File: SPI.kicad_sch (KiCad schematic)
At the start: 1 part, among them J14 Conn_01x08

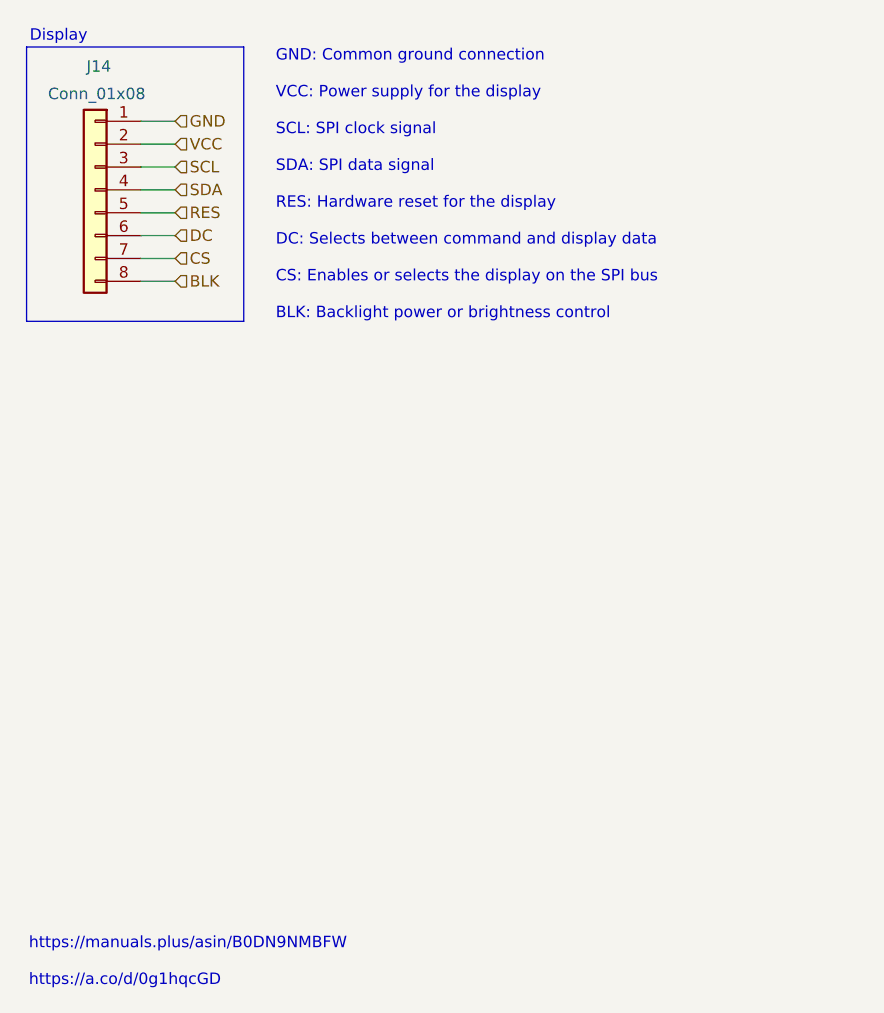
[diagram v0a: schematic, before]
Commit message: org stuf
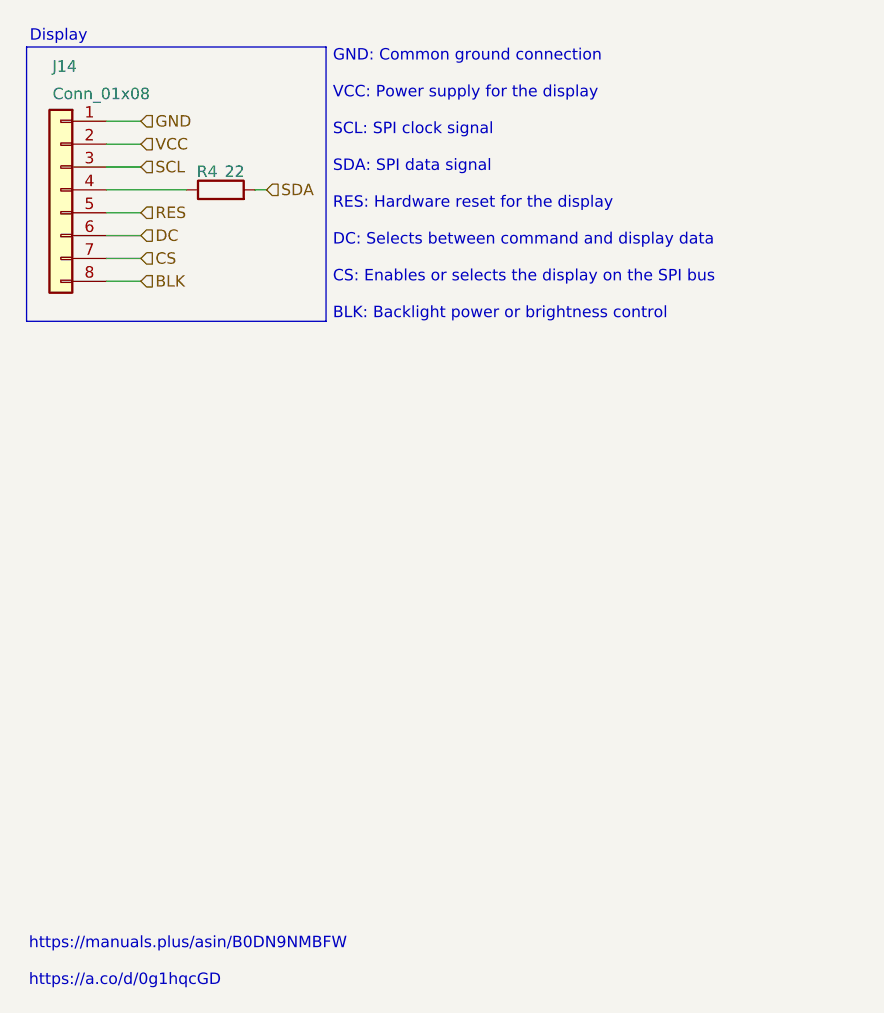
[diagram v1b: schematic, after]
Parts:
- added R4: 22, symbol Device:R
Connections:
- net SDA: now also R4.2; no longer J14.4 (Pin_4)
- new net: J14.4 (Pin_4), R4.1
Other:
- moved on the sheet: J14
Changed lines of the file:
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@@
 	(rectangle
 		(start 15.24 15.875)
-		(end 39.37 46.355)
+		(end 48.514 46.355)
 		(stroke
 			(width 0)
@@
 	(text "GND: Common ground connection\n\nVCC: Power supply for the display\n\nSCL: SPI clock signal\n\nSDA: SPI data signal\n\nRES: Hardware reset for the display\n\nDC: Selects between command and display data\n\nCS: Enables or selects the display on the SPI bus\n\nBLK: Backlight power or brightness control"
 		(exclude_from_sim no)
-		(at 42.926 31.242 0)
+		(at 49.276 31.242 0)
 		(effects
 			(font
@@
 	(wire
 		(pts
-			(xy 27.94 29.21) (xy 31.75 29.21)
+			(xy 24.13 29.21) (xy 27.94 29.21)
 		)
 		(stroke
@@
 	(wire
 		(pts
-			(xy 27.94 24.13) (xy 31.75 24.13)
+			(xy 24.13 24.13) (xy 27.94 24.13)
 		)
 		(stroke
@@
 	(wire
 		(pts
-			(xy 27.94 34.29) (xy 31.75 34.29)
+			(xy 24.13 34.29) (xy 27.94 34.29)
 		)
 		(stroke
@@
 	(wire
 		(pts
-			(xy 27.94 26.67) (xy 31.75 26.67)
+			(xy 24.13 26.67) (xy 27.94 26.67)
 		)
 		(stroke
@@
 	(wire
 		(pts
-			(xy 27.94 31.75) (xy 31.75 31.75)
+			(xy 24.13 31.75) (xy 33.02 31.75)
 		)
 		(stroke
@@
 	(wire
 		(pts
-			(xy 27.94 39.37) (xy 31.75 39.37)
+			(xy 24.13 39.37) (xy 27.94 39.37)
 		)
 		(stroke
@@
 	(wire
 		(pts
-			(xy 27.94 36.83) (xy 31.75 36.83)
+			(xy 24.13 36.83) (xy 27.94 36.83)
 		)
 		(stroke
@@
 	(wire
 		(pts
-			(xy 27.94 41.91) (xy 31.75 41.91)
+			(xy 40.64 31.75) (xy 41.91 31.75)
+		)
+		(stroke
+			(width 0)
+			(type default)
+		)
+	)
+	(wire
+		(pts
+			(xy 24.13 41.91) (xy 27.94 41.91)
 		)
 		(stroke
@@
 	(hierarchical_label "RES"
 		(shape input)
-		(at 31.75 34.29 0)
+		(at 27.94 34.29 0)
 		(effects
 			(font
@@
 	(hierarchical_label "VCC"
 		(shape input)
-		(at 31.75 26.67 0)
+		(at 27.94 26.67 0)
 		(effects
 			(font
@@
 	(hierarchical_label "GND"
 		(shape input)
-		(at 31.75 24.13 0)
+		(at 27.94 24.13 0)
 		(effects
 			(font
@@
 	(hierarchical_label "SCL"
 		(shape input)
-		(at 31.75 29.21 0)
+		(at 27.94 29.21 0)
 		(effects
 			(font
@@
 	(hierarchical_label "DC"
 		(shape input)
-		(at 31.75 36.83 0)
+		(at 27.94 36.83 0)
 		(effects
 			(font
@@
 	(hierarchical_label "CS"
 		(shape input)
-		(at 31.75 39.37 0)
+		(at 27.94 39.37 0)
 		(effects
 			(font
@@
 	(hierarchical_label "SDA"
 		(shape input)
-		(at 31.75 31.75 0)
+		(at 41.91 31.75 0)
 		(effects
 			(font
@@
 	(hierarchical_label "BLK"
 		(shape input)
-		(at 31.75 41.91 0)
+		(at 27.94 41.91 0)
 		(effects
 			(font
@@
 	(symbol
 		(lib_id "Connector_Generic:Conn_01x08")
-		(at 22.86 31.75 0)
+		(at 19.05 31.75 0)
 		(mirror y)
 		(unit 1)
@@
 		(dnp no)
 		(property "Reference" "J14"
-			(at 24.638 18.034 0)
+			(at 20.828 18.034 0)
 			(show_name no)
 			(do_not_autoplace no)
@@
 		)
 		(property "Value" "Conn_01x08"
-			(at 28.448 21.082 0)
+			(at 28.956 21.082 0)
 			(show_name no)
 			(do_not_autoplace no)
@@
 		)
 		(property "Footprint" "Package_DIP:DIP-20_W7.62mm"
-			(at 22.86 31.75 0)
+			(at 19.05 31.75 0)
 			(hide yes)
 			(show_name no)
@@
 		)
 		(property "Datasheet" "kicad-embed://ST7789V.pdf"
-			(at 22.86 31.75 0)
+			(at 19.05 31.75 0)
 			(hide yes)
 			(show_name no)
@@
 		)
 		(property "Description" "Generic connector, single row, 01x08, script generated (kicad-library-utils/schlib/autogen/connector/)"
-			(at 22.86 31.75 0)
+			(at 19.05 31.75 0)
 			(hide yes)
 			(show_name no)
@@
 					(unit 1)
 				)
+			)
+		)
+	)
+	(symbol
+		(lib_id "Device:R")
+		(at 36.83 31.75 90)
+		(unit 1)
+		(body_style 1)
+		(exclude_from_sim no)
+		(in_bom yes)
+		(on_board yes)
+		(in_pos_files yes)
+		(dnp no)
+		(property "Reference" "R4"
+			(at 35.306 29.718 90)
+			(show_name no)
+			(do_not_autoplace no)
+			(effects
+				(font
+					(size 1.27 1.27)
+				)
+			)
+		)
+		(property "Value" "22"
+			(at 38.354 29.718 90)
+			(show_name no)
+			(do_not_autoplace no)
+			(effects
+				(font
+					(size 1.27 1.27)
+				)
+			)
+		)
+		(property "Footprint" ""
+			(at 36.83 33.528 90)
+			(hide yes)
+			(show_name no)
+			(do_not_autoplace no)
+			(effects
+				(font
+					(size 1.27 1.27)
+				)
+			)
+		)
+		(property "Datasheet" ""
+			(at 36.83 31.75 0)
+			(hide yes)
+			(show_name no)
+			(do_not_autoplace no)
+			(effects
+				(font
+					(size 1.27 1.27)
+				)
+			)
+		)
+		(property "Description" "Resistor"
+			(at 36.83 31.75 0)
+			(hide yes)
+			(show_name no)
+			(do_not_autoplace no)
+			(effects
+				(font
+					(size 1.27 1.27)
+				)
+			)
+		)
+		(pin "2"
+		)
+		(pin "1"
+		)
+		(instances
+			(project "PS-ChargerInterfacePCB"
+				(path "/894adbd2-6316-426a-afb4-88808e8ec51a/d8590700-a995-4af9-a193-f270d7e0e413"
+					(reference "R4")
+					(unit 1)
+				)

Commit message: final schem is done
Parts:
- R4: footprint (none) -> Resistor_SMD:R_0603_1608Metric_Pad0.98x0.95mm_HandSolder
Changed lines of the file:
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@@
 			)
 		)
-		(property "Footprint" ""
+		(property "Footprint" "Resistor_SMD:R_0603_1608Metric_Pad0.98x0.95mm_HandSolder"
 			(at 36.83 33.528 90)
 			(hide yes)

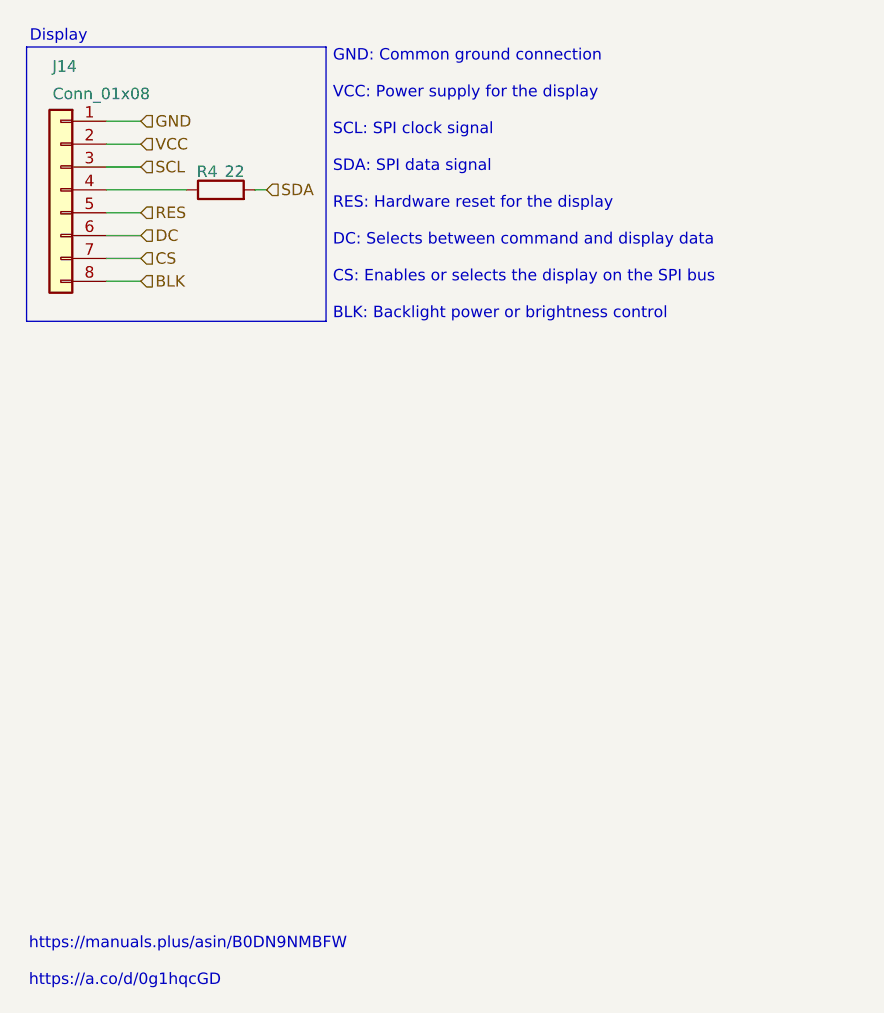
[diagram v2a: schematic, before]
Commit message: shoupu review done
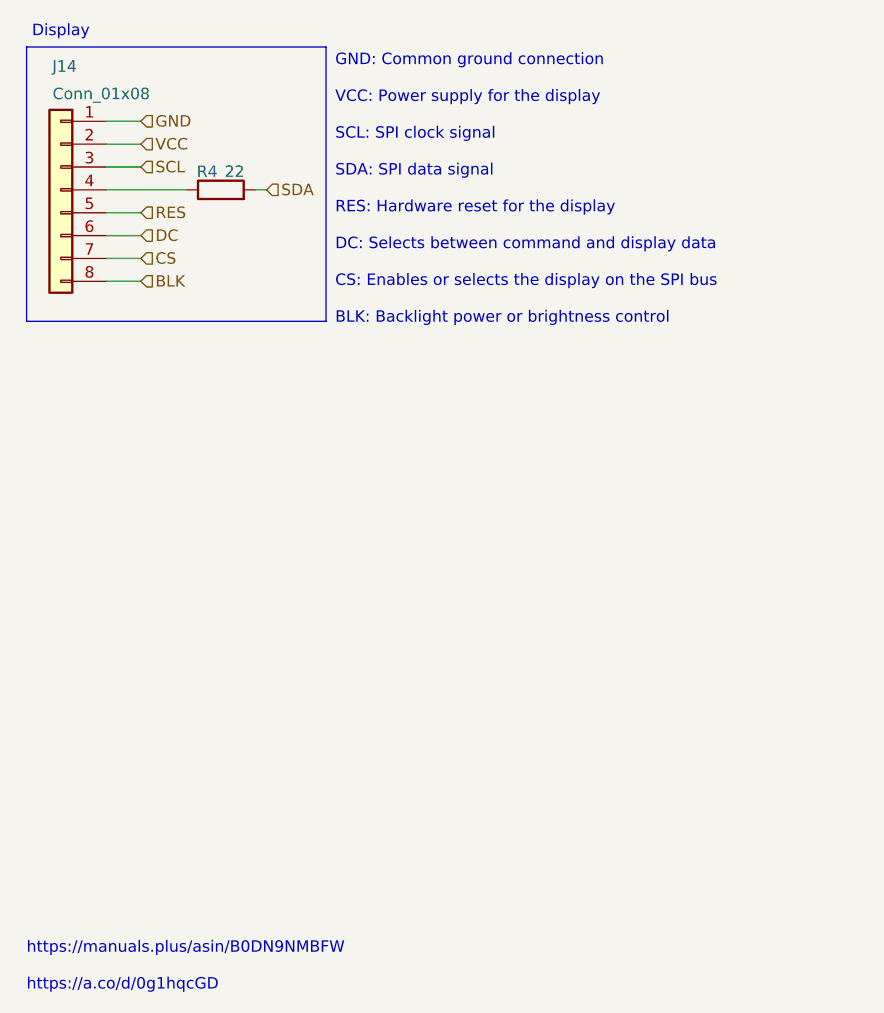
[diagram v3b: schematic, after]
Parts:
- J14: footprint Package_DIP:DIP-20_W7.62mm -> Connector_PinSocket_2.54mm:PinSocket_1x08_P2.54mm_Vertical
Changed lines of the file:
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@@
 	(text "GND: Common ground connection\n\nVCC: Power supply for the display\n\nSCL: SPI clock signal\n\nSDA: SPI data signal\n\nRES: Hardware reset for the display\n\nDC: Selects between command and display data\n\nCS: Enables or selects the display on the SPI bus\n\nBLK: Backlight power or brightness control"
 		(exclude_from_sim no)
-		(at 49.276 31.242 0)
+		(at 49.53 31.75 0)
 		(effects
 			(font
@@
 	(text "Display\n\n"
 		(exclude_from_sim no)
-		(at 18.796 15.748 0)
+		(at 19.05 15.24 0)
 		(effects
 			(font
@@
 	(text "https://manuals.plus/asin/B0DN9NMBFW\n\nhttps://a.co/d/0g1hqcGD"
 		(exclude_from_sim no)
-		(at 15.494 117.602 0)
+		(at 15.24 118.11 0)
 		(effects
 			(font
@@
 			)
 		)
-		(property "Footprint" "Package_DIP:DIP-20_W7.62mm"
+		(property "Footprint" "Connector_PinSocket_2.54mm:PinSocket_1x08_P2.54mm_Vertical"
 			(at 19.05 31.75 0)
 			(hide yes)
